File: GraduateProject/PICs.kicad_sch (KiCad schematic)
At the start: 28 parts, among them IC1 PIC16C620A-04/SS, IC2 PIC16C620A-04/SS, Q1 BST50,115, SW1 SS12D10G3

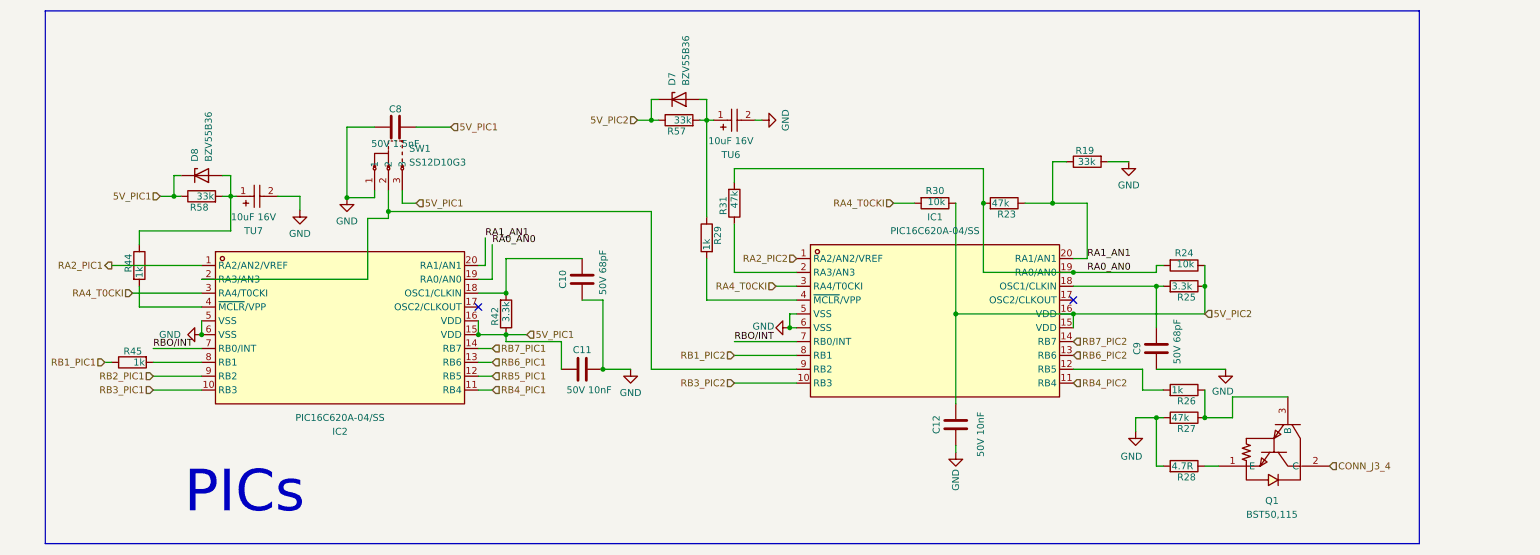
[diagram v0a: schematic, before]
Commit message: 3/9/25
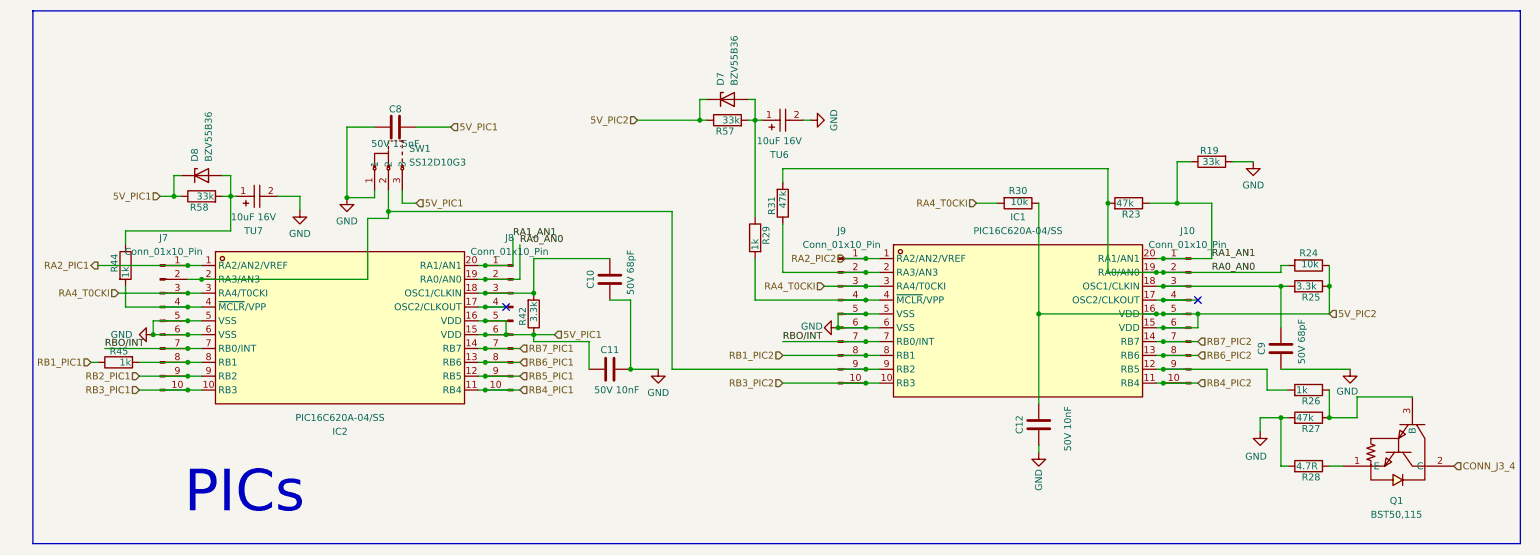
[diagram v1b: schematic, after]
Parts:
- added J10, J7, J8, J9: Conn_01x10_Pin, symbol Connector:Conn_01x10_Pin
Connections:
- net 5V_PIC1: now also J8.5 (Pin_5), J8.6 (Pin_6)
- net 5V_PIC2: now also J10.5 (Pin_5), J10.6 (Pin_6)
- net GND: now also J7.5 (Pin_5), J7.6 (Pin_6), J9.5 (Pin_5), J9.6 (Pin_6)
- net RA0_AN0: now also J10.2 (Pin_2), J8.2 (Pin_2)
- net RA1_AN1: now also J10.1 (Pin_1), J8.1 (Pin_1)
- net RA2_PIC1: now also J7.1 (Pin_1)
- net RA2_PIC2: now also J9.1 (Pin_1)
- net RA4_T0CKI: now also J7.3 (Pin_3), J9.3 (Pin_3)
- net RB1_PIC2: now also J9.8 (Pin_8)
- net RB2_PIC1: now also J7.9 (Pin_9)
- net RB3_PIC1: now also J7.10 (Pin_10)
- net RB3_PIC2: now also J9.10 (Pin_10)
- net RB4_PIC1: now also J8.10 (Pin_10)
- net RB4_PIC2: now also J10.10 (Pin_10)
- net RB5_PIC1: now also J8.9 (Pin_9)
- net RB6_PIC1: now also J8.8 (Pin_8)
- net RB6_PIC2: now also J10.8 (Pin_8)
- net RB7_PIC1: now also J8.7 (Pin_7)
- net RB7_PIC2: now also J10.7 (Pin_7)
- net RBO/INT: now also J7.7 (Pin_7), J9.7 (Pin_7)
- net at C9.1, IC1.18 (OSC1/CLKIN), R25.2: now also J10.3 (Pin_3)
- net at IC1.4 (~{MCLR}/VPP), R29.2: now also J9.4 (Pin_4)
- net at IC1.9 (RB2), IC2.2 (RA3/AN3), SW1.2: now also J7.2 (Pin_2), J9.9 (Pin_9)
- net at IC2.8 (RB1), R45.2: now also J7.8 (Pin_8)
- net at C10.1, IC2.18 (OSC1/CLKIN), R42.2: now also J8.3 (Pin_3)
- net at IC2.17 (OSC2/CLKOUT): now also J8.4 (Pin_4)
- net at IC2.4 (~{MCLR}/VPP), R44.2: now also J7.4 (Pin_4)
- net at IC1.12 (RB5), R26.2: now also J10.9 (Pin_9)
- net at IC1.17 (OSC2/CLKOUT): now also J10.4 (Pin_4)
- net at IC1.2 (RA3/AN3), R31.1: now also J9.2 (Pin_2)
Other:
- moved on the sheet: C10, C11, C12, C9, D7, IC1, Q1, R19, R23, R24, R25, R26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

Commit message: Add files via upload
10/9/25
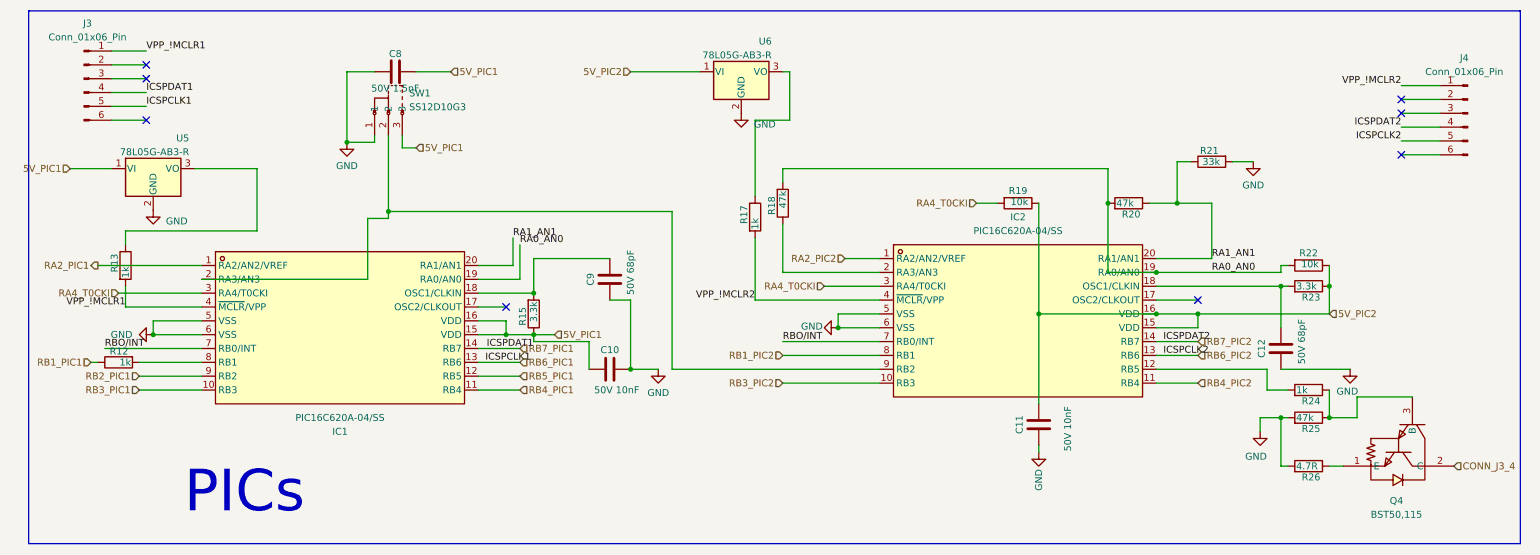
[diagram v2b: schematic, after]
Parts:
- removed D7, D8: BZV55B36, Diode_SMD:D_MiniMELF, symbol Diode:BZV55B36
- removed J10, J7, J8, J9: Conn_01x10_Pin, symbol Connector:Conn_01x10_Pin
- removed R57, R58: 33k, Resistor_SMD:R_0805_2012Metric, symbol Device:R
- removed TU6, TU7: 10uF 16V, easyeda2kicad:CAP-SMD_L3.2-W1.6-RD-C7171, symbol easyeda2kicad:TAJA106K016RNJ
- added J3, J4: Conn_01x06_Pin, Connector_PinHeader_2.54mm:PinHeader_1x06_P2.54mm_Vertical, symbol Connector:Conn_01x06_Pin
- added U5, U6: 78L05G-AB3-R, Package_TO_SOT_SMD:SOT-89-3, symbol Regulator_Linear:KA78M05_TO252
- renumbered C11 to C10, C12 to C11, C9 to C12, C10 to C9, IC2 to IC1, IC1 to IC2, Q1 to Q4, R45 to R12, R44 to R13, R42 to R15, R29 to R17, R31 to R18, R30 to R19, R23 to R20, R19 to R21, R24 to R22, R25 to R23, R26 to R24, R27 to R25, R28 to R26
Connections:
- net 5V_PIC1: now also U5.1 (VI)
- net 5V_PIC2: now also U6.1 (VI)
- net GND: now also U5.2 (GND), U6.2 (GND)
- net RB6_PIC1: now also J3.5 (Pin_5)
- net RB6_PIC2: now also J4.5 (Pin_5)
- net RB7_PIC1: now also J3.4 (Pin_4)
- net RB7_PIC2: now also J4.4 (Pin_4)
- net at R13.1: now also U5.3 (VO)
- net at R17.1: now also U6.3 (VO)
- net VPP_!MCLR2: now reaches IC2.4 (~{MCLR}/VPP), R17.2
- net VPP_!MCLR2: now also J4.1 (Pin_1)
- net VPP_!MCLR1: now reaches IC1.4 (~{MCLR}/VPP), R13.2
- net VPP_!MCLR1: now also J3.1 (Pin_1)
- no-connect marks 2 -> 8
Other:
- moved on the sheet: C8, R17, SW1

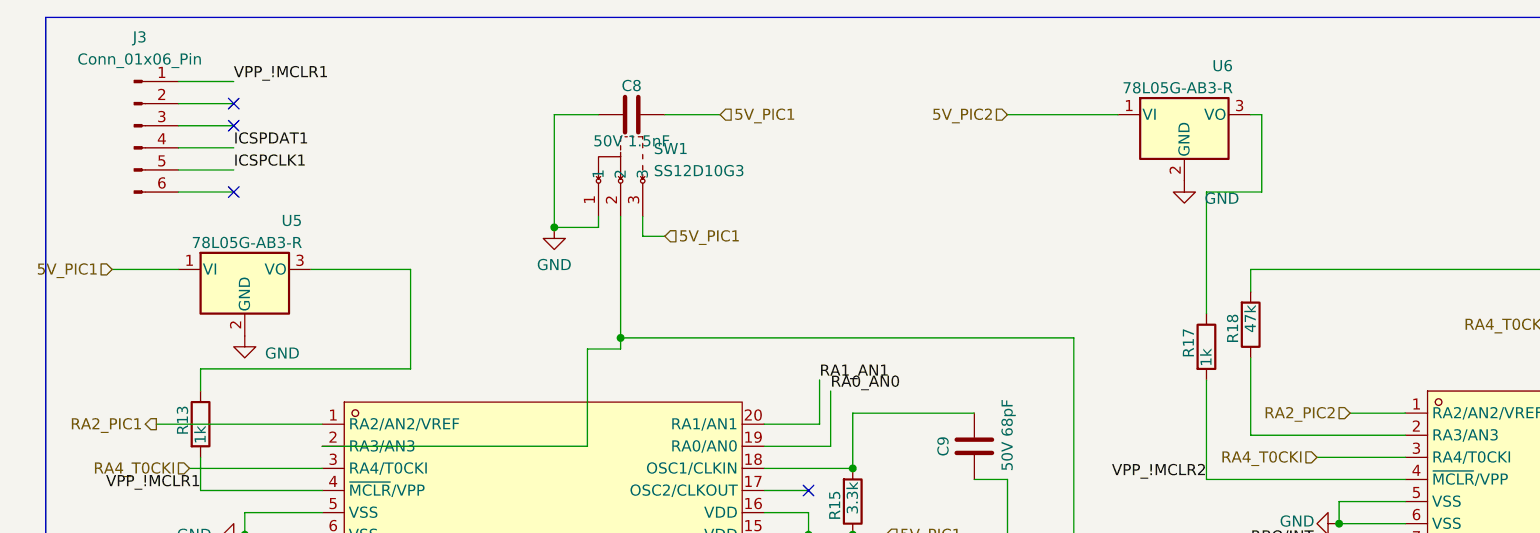
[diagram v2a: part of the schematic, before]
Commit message: Add files via upload
Add BOM
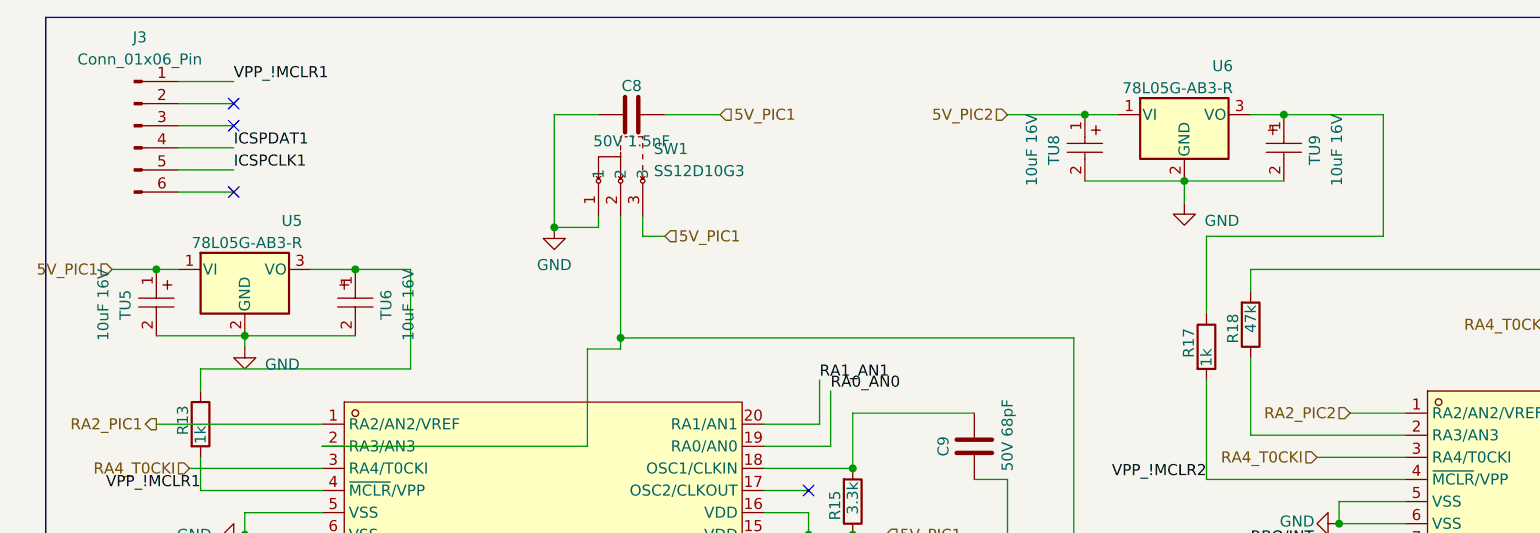
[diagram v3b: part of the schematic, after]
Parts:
- added TU5, TU6, TU8, TU9: 10uF 16V, easyeda2kicad:CAP-SMD_L3.2-W1.6-RD-C7171, symbol easyeda2kicad:TAJA106K016RNJ
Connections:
- net 5V_PIC1: now also TU5.1
- net 5V_PIC2: now also TU8.1
- net GND: now also TU5.2, TU6.2, TU8.2, TU9.2
- net at R17.1, U6.3 (VO): now also TU9.1
- net at R13.1, U5.3 (VO): now also TU6.1
